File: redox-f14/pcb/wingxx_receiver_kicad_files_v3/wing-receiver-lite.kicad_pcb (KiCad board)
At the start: 2 copper layers, 22.6 x 43.9 mm, 27 parts, among them U1 ATmega32U4-AU, X1 Crystal_GND24

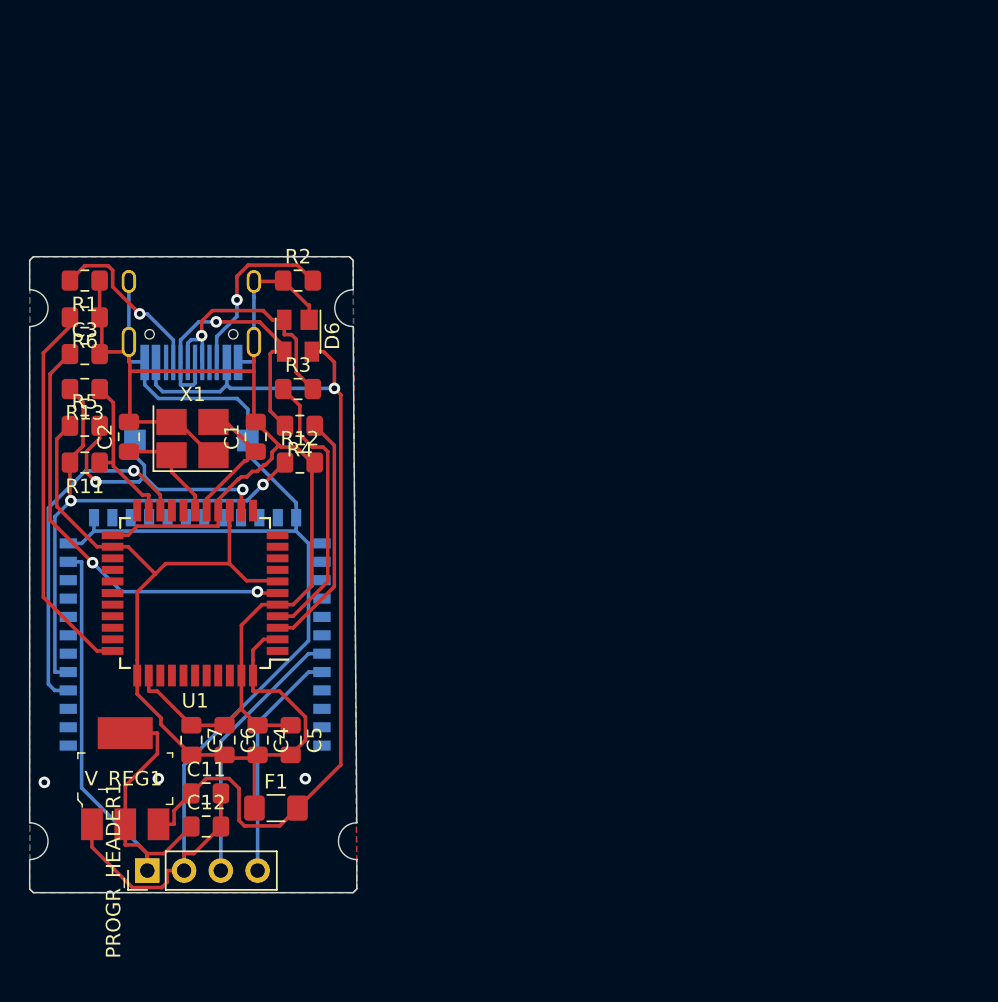
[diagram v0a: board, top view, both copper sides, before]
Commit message: update to new style
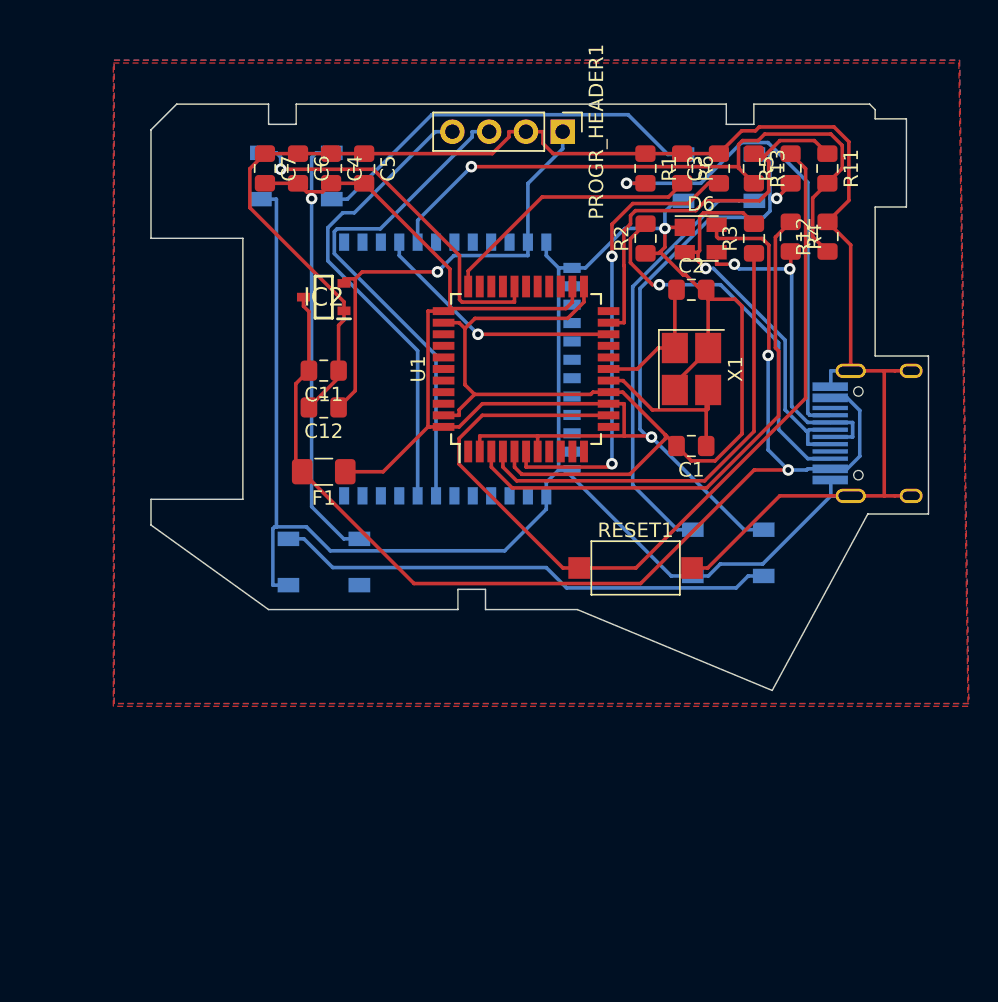
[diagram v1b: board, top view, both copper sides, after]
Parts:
- removed V_REG1: LD1117S33CTR, redox_w_receiver_footprints:SOT-223
- added D1: WS2812B, LED_SMD:LED_WS2812B_PLCC4_5.0x5.0mm_P3.2mm, B.Cu at (87.0, 87.4)
- added D2: WS2812B, LED_SMD:LED_WS2812B_PLCC4_5.0x5.0mm_P3.2mm, B.Cu at (116.2, 87.5)
- added D3: WS2812B, LED_SMD:LED_WS2812B_PLCC4_5.0x5.0mm_P3.2mm, B.Cu at (116.8, 113.4)
- added D4: WS2812B, LED_SMD:LED_WS2812B_PLCC4_5.0x5.0mm_P3.2mm, B.Cu at (88.9, 114.1)
- added IC2: XC6206P332MR, XC6206P332MR:SOT95P280X130-3N, F.Cu at (88.9, 95.8)
- C11, C12: value 10uF -> 1uF
- RESET1: moved to F.Cu
- moved PROGR_HEADER1 58.6 mm to (105.4, 84.3), turned to 270 degrees
- moved R11 55.2 mm to (123.7, 86.9), turned to 270 degrees
- moved USB1 53.9 mm to (132.1, 105.2), turned to 270 degrees
- moved R5 51.9 mm to (121.2, 86.9), turned to 90 degrees
- moved R13 48.7 mm to (118.6, 86.9), turned to 270 degrees
- moved C3 45.7 mm to (116.2, 86.9), turned to 90 degrees
- moved R6 42.5 mm to (113.7, 86.9), turned to 270 degrees
- moved C2 40.2 mm to (114.3, 95.2), turned to 0 degrees
- moved C4 39.8 mm to (89.4, 86.9)
- moved C5 39.8 mm to (91.7, 86.9)
- moved C6 39.8 mm to (87.1, 86.9)
- moved C7 39.8 mm to (84.8, 86.9)
- moved R12 39.7 mm to (123.7, 91.6), turned to 90 degrees
- moved R1 39.5 mm to (111.1, 86.9), turned to 270 degrees
- moved R4 36.3 mm to (121.2, 91.6), turned to 270 degrees
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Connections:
- C11 pad 1: VCC -> GND
- C11 pad 2: GND -> VCC
- U1 pad 29: Net-(U1-Pad29) -> P5
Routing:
- net GND: track 187.6 -> 303.4 mm, vias 3 -> 1
- net +5V: track 65.0 -> 144.9 mm, vias 0 -> 3
- net Net-(R5-Pad2): track 19.4 -> 61.9 mm, vias 2 -> 0
- net Net-(D3-Pad2): track 0.00 -> 34.6 mm
- net Net-(D2-Pad2): track 0.00 -> 30.0 mm
- net Net-(D1-Pad2): track 0.00 -> 27.9 mm
- net P5: track 0.00 -> 25.1 mm, vias 0 -> 1
- net Net-(R1-Pad2): track 11.9 -> 33.7 mm
- net D-: track 16.8 -> 37.5 mm
- net VCC: track 64.6 -> 84.5 mm, vias 1 -> 2
- net SWDIO: track 18.4 -> 34.9 mm
- net TXO: track 11.0 -> 27.5 mm
- net SWCLK: track 16.1 -> 32.5 mm
- net Net-(R2-Pad2): track 12.5 -> 26.1 mm
- net D+: track 19.5 -> 32.5 mm
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- added copper zone on F.Cu, net (none)
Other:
- board size 22.6 x 43.9 mm -> 53.7 x 40.5 mm
